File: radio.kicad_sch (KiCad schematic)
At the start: 36 parts, among them Q1 BSS138W-7-F, U2 SX1276IMLTRT, U3 SX1276IMLTRT, X1 AS183-92LF, Y1 ECS-TXO-25CSMV-320-AM-TR

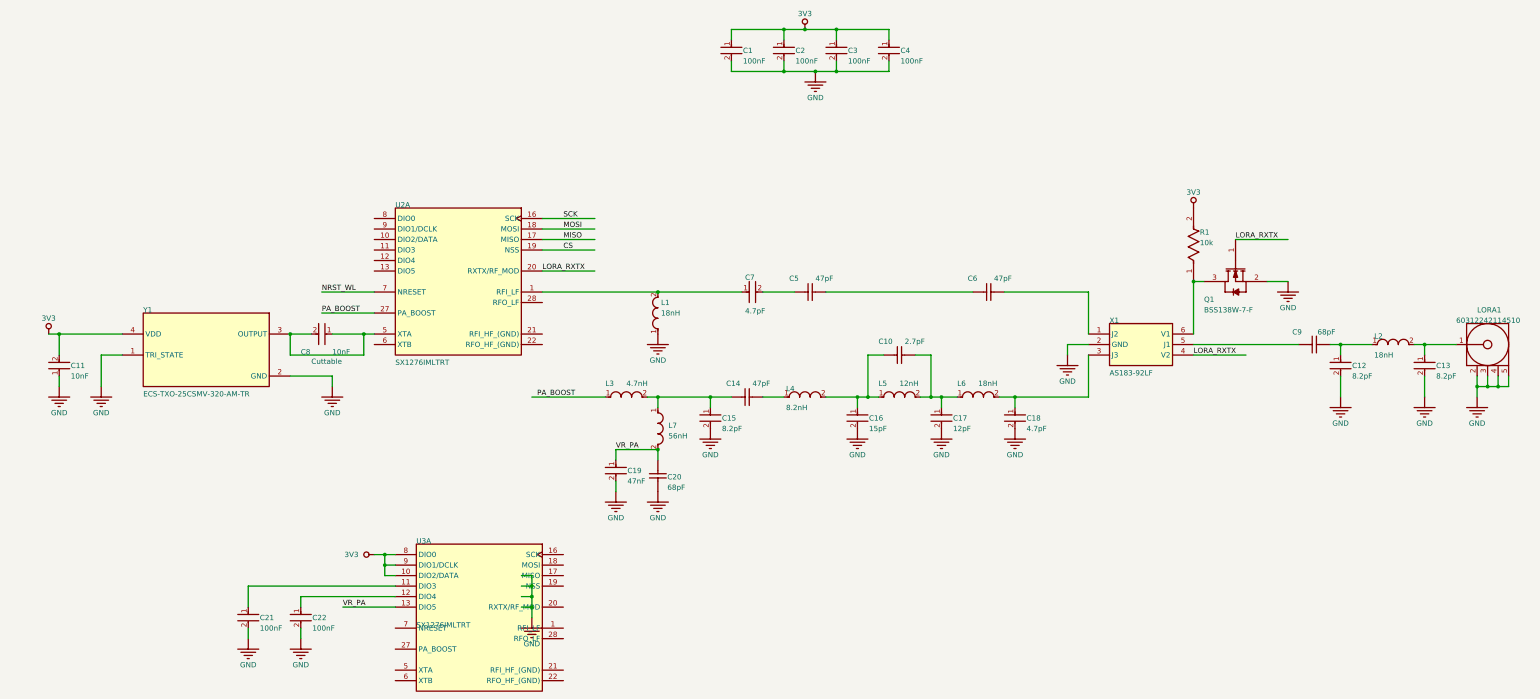
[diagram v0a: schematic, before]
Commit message: fix sx1276
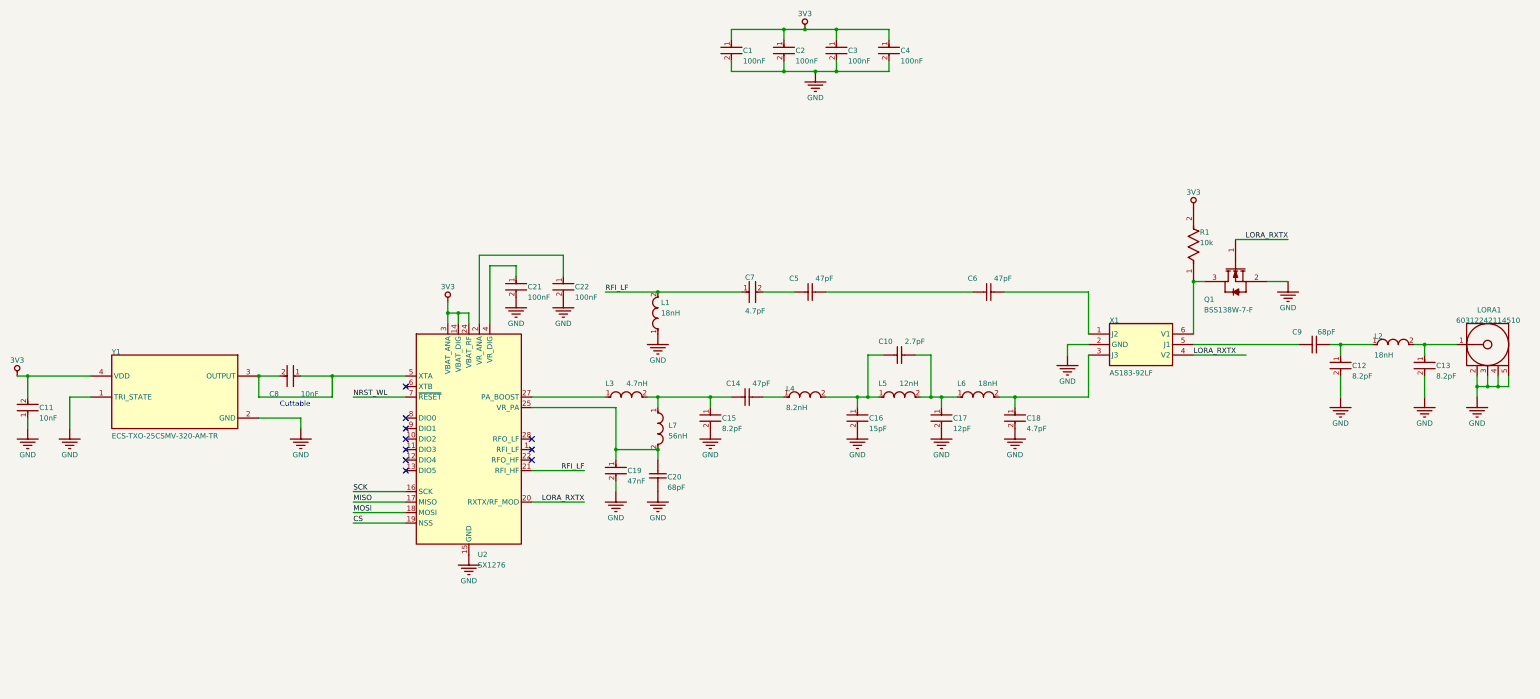
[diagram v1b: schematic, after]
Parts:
- removed C21: 100nF, FP-C0603C-CF-MFG, symbol Altium Content Vault:root_0_b4654b650e69147ec39a6b967a45e02_Altium Content Vault
- removed U2, U3: SX1276IMLTRT, SMTC-QFN-28_V, symbol Altium Content Vault:root_0_SMTC-SX127X-QFN-28_Altium Content Vault
- added U2: SX1276, Package_DFN_QFN:QFN-28-1EP_6x6mm_P0.65mm_EP4.8x4.8mm, symbol RF:SX1276
- renumbered C1 to C21
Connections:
- net 3V3: now also U2.14 (VBAT_DIG), U2.24 (VBAT_RF), U2.3 (VBAT_ANA)
- net CS: now also U2.19 (NSS)
- net GND: now also U2.15 (GND), U2.23 (GND), U2.26 (GND), U2.29 (GND)
- net LORA_RXTX: now also U2.20 (RXTX/RF_MOD)
- net MISO: now also U2.17 (MISO)
- net MOSI: now also U2.18 (MOSI)
- net NRST_WL: now also U2.7 (~{RESET})
- net SCK: now also U2.16 (SCK)
- net at C22.1: now also U2.2 (VR_ANA)
- net RFI_LF: now reaches C7.1, L1.2
- net RFI_LF: now also U2.21 (RFI_HF)
- net at C8.1, C8.2, Y1.3 (OUTPUT): now also U2.5 (XTA)
- net PA_BOOST: no longer names the net of L3.1
- net PA_BOOST: now also U2.27 (PA_BOOST)
- net VR_PA: no longer names the net of C19.1, C20.2, L7.2
- net VR_PA: now also U2.25 (VR_PA)
- new net: C21.1, U2.4 (VR_DIG)
- no-connect marks 0 -> 10
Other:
- moved on the sheet: C11, C8, Y1
